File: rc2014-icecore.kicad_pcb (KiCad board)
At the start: 2 copper layers, 70.3 x 60.7 mm, 7 parts, among them J1 Conn_02x25_Odd_Even, J2 Conn_02x15_Odd_Even, J3 Conn_02x13_Odd_Even

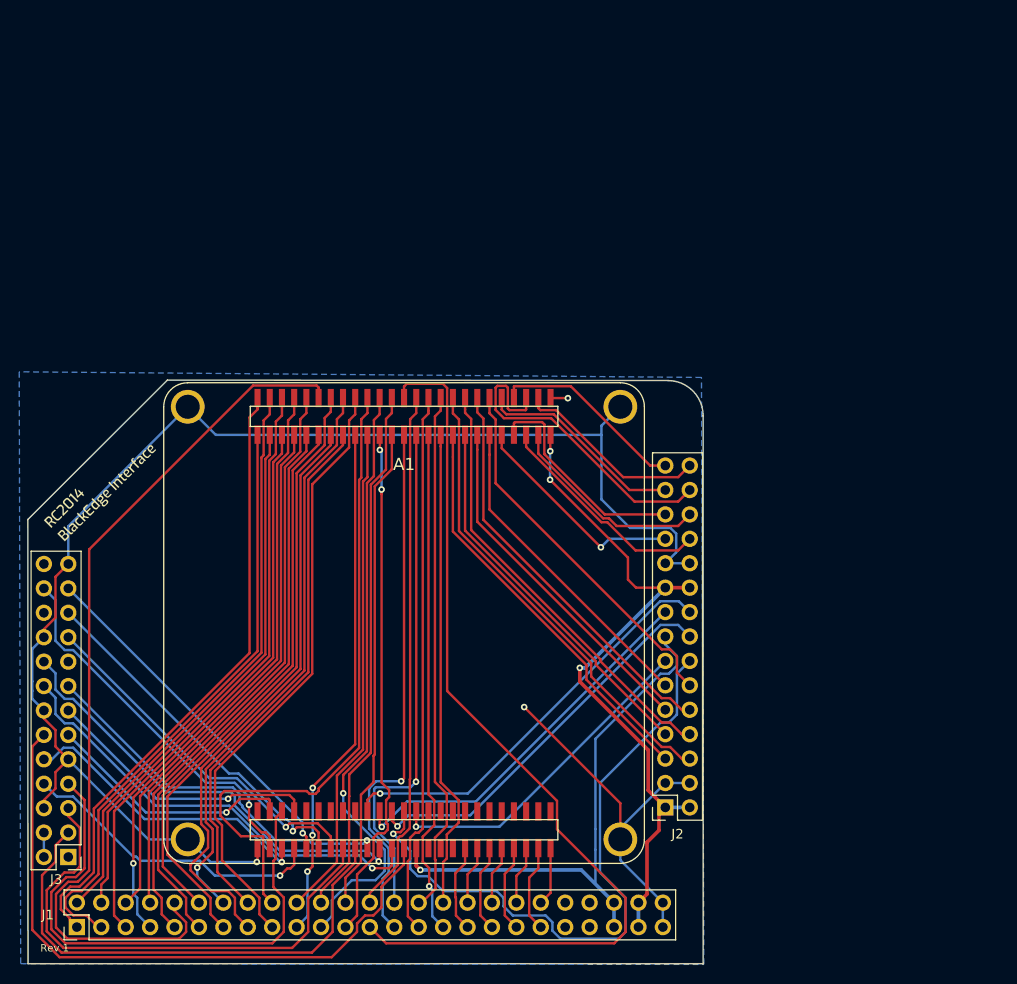
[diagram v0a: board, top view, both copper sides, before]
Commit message: Start new merged design
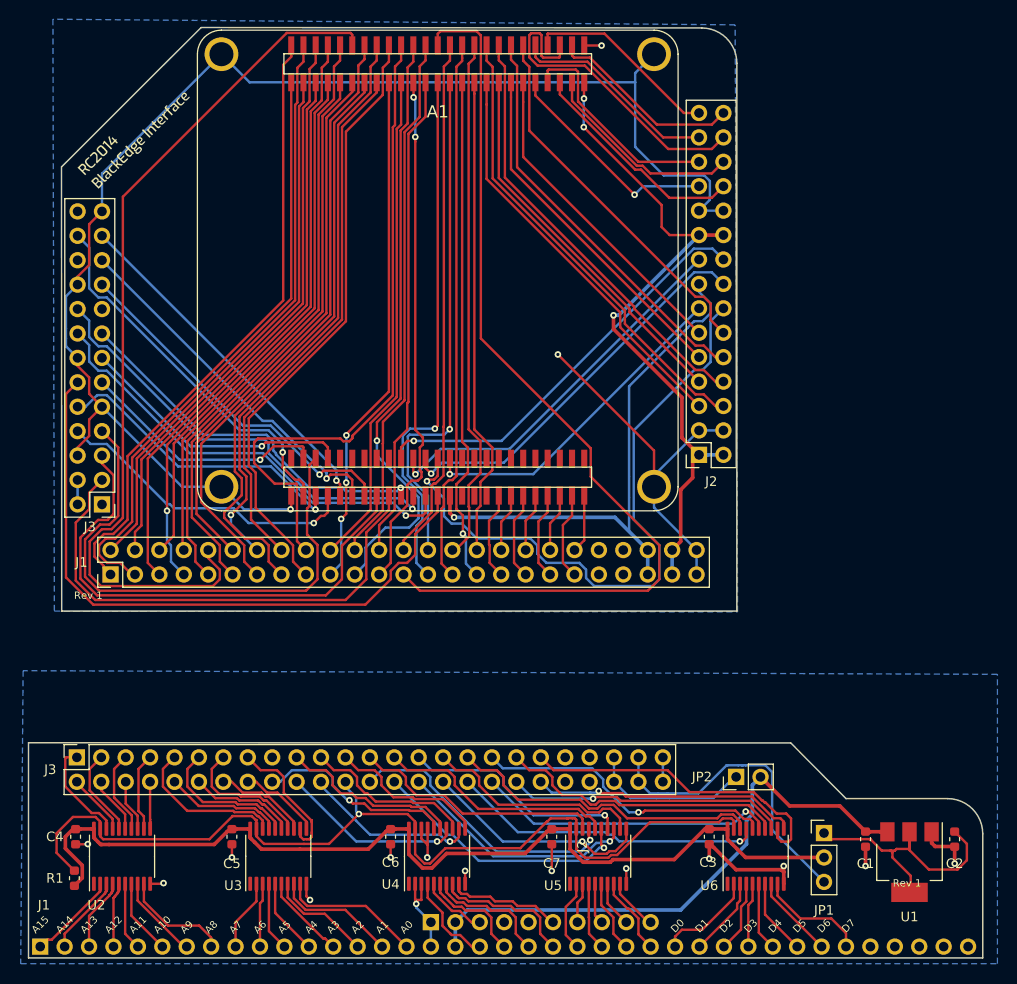
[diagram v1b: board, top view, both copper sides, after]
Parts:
- added C1: 100nF, Capacitor_SMD:C_0603_1608Metric, F.Cu at (147.6, 152.1)
- added C2: 10uF, Capacitor_SMD:C_0603_1608Metric, F.Cu at (156.8, 152.1)
- added C3: C, Capacitor_SMD:C_0603_1608Metric, F.Cu at (131.3, 151.9)
- added C4: C, Capacitor_SMD:C_0603_1608Metric, F.Cu at (65.4, 151.9)
- added C5: C, Capacitor_SMD:C_0603_1608Metric, F.Cu at (81.7, 151.9)
- added C6: C, Capacitor_SMD:C_0603_1608Metric, F.Cu at (98.2, 151.9)
- added C7: C, Capacitor_SMD:C_0603_1608Metric, F.Cu at (114.9, 151.9)
- added J1: Conn_01x39, rc2014:PinHeader_1x39_P2.54mm_Vertical_NoSilk, F.Cu at (61.7, 163.3)
- added J2: Conn_01x10, rc2014:PinHeader_1x10_P2.54mm_Vertical_NoSilk, F.Cu at (102.4, 160.8)
- added J3: Conn_02x25_Odd_Even, Connector_PinSocket_2.54mm:PinSocket_2x25_P2.54mm_Vertical, F.Cu at (65.5, 143.6)
- added JP1: Ext Power, Connector_PinHeader_2.54mm:PinHeader_1x03_P2.54mm_Vertical, F.Cu at (143.3, 151.5)
- added JP2: Jumper, Connector_PinHeader_2.54mm:PinHeader_1x02_P2.54mm_Vertical, F.Cu at (134.1, 145.7)
- added R1: R, Resistor_SMD:R_0603_1608Metric, F.Cu at (65.3, 156.2)
- added REF**: OSHW-Symbol_6.7x6mm_SilkScreen, Symbol:OSHW-Symbol_6.7x6mm_SilkScreen, B.Cu at (152.4, 155.2)
- added U1: LM1117-3.3, Package_TO_SOT_SMD:SOT-223-3_TabPin2, F.Cu at (152.1, 154.5)
- added U2: SN74CB3T3245, Package_SO:TSSOP-20_4.4x6.5mm_P0.65mm, F.Cu at (70.2, 153.9)
- added U3: SN74CB3T3245, Package_SO:TSSOP-20_4.4x6.5mm_P0.65mm, F.Cu at (86.5, 153.9)
- added U4: SN74CB3T3245, Package_SO:TSSOP-20_4.4x6.5mm_P0.65mm, F.Cu at (103.0, 153.9)
- added U5: SN74CB3T3245, Package_SO:TSSOP-20_4.4x6.5mm_P0.65mm, F.Cu at (119.8, 153.9)
- added U6: SN74CB3T3245, Package_SO:TSSOP-20_4.4x6.5mm_P0.65mm, F.Cu at (136.1, 153.9)
- moved A1 36.8 mm to (87.8, 69.5)
- moved G*** 36.8 mm to (71.4, 78.6)
- moved G*** 36.8 mm to (105.3, 89.5)
- moved J1 36.8 mm to (69.0, 124.6)
- moved J2 36.8 mm to (130.3, 112.2)
- moved J3 36.8 mm to (68.1, 117.3)
- moved REF** 36.8 mm to (119.8, 104.9)
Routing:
- net +3V3: track 0.00 -> 100.5 mm
- net /P23: track 50.7 -> 148.9 mm, vias 0 -> 1
- net +5V: track 59.6 -> 118.9 mm
- net GND: track 187.6 -> 237.4 mm, vias 3 -> 17
- net /P54: track 9.11 -> 42.6 mm
- net /P48: track 9.16 -> 42.2 mm
- net /P49: track 6.10 -> 38.7 mm, vias 0 -> 1
- net /FPGA_VCC: track 71.9 -> 104.0 mm
- net /P51: track 6.10 -> 37.4 mm, vias 0 -> 1
- net /P50: track 9.11 -> 40.3 mm, vias 0 -> 1
- net /P52: track 9.11 -> 39.3 mm
- net Net-(C2-Pad1): track 0.00 -> 29.4 mm
- net /P25: track 54.6 -> 83.9 mm, vias 0 -> 1
- net /P53: track 6.10 -> 35.2 mm, vias 0 -> 1
- net /P27: track 53.5 -> 81.4 mm, vias 1 -> 2
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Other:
- board size 70.3 x 60.7 mm -> 99.3 x 96.8 mm
- board text added: "+5V"
- board text added: "2018, 2020 Ed Brindley"
- board text added: "A0"
- board text added: "A1"
- board text added: "A10"
- board text added: "A11"
- board text added: "A12"
- board text added: "A13"
- board text added: "A14"
- board text added: "A15"
- board text added: "A2"
- board text added: "A3"
- board text added: "A4"
- board text added: "A5"
- board text added: "A6"
- board text added: "A7"
- board text added: "A8"
- board text added: "A9"
- board text added: "CLK/NC"
- board text added: "D0"
- board text added: "D1"
- board text added: "D2"
- board text added: "D3"
- board text added: "D4"
- board text added: "D5"
- board text added: "D6"
- board text added: "D7"
- board text added: "GND"
- board text added: "INT/BUSACK"
- board text added: "IORQ/NMI"
- board text added: "M1/RFSH"
- board text added: "MRQ/HALT"
- board text added: "RD/WAIT"
- board text added: "RST/NC"
- board text added: "SN74CB3T3245 FPGA Level Translator"
- board text added: "WR/NC"
